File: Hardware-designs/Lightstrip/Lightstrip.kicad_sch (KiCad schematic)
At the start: 22 parts, among them J1 In 24V, J2 lamps, J3 UART, Q1 AO3400A, SW1 PTS526 SM15 SMTR2 LFS, SW2 PTS526 SM15 SMTR2 LFS, U1 TPS560430X3FDBVT, U2 ESP32-WROOM-32E

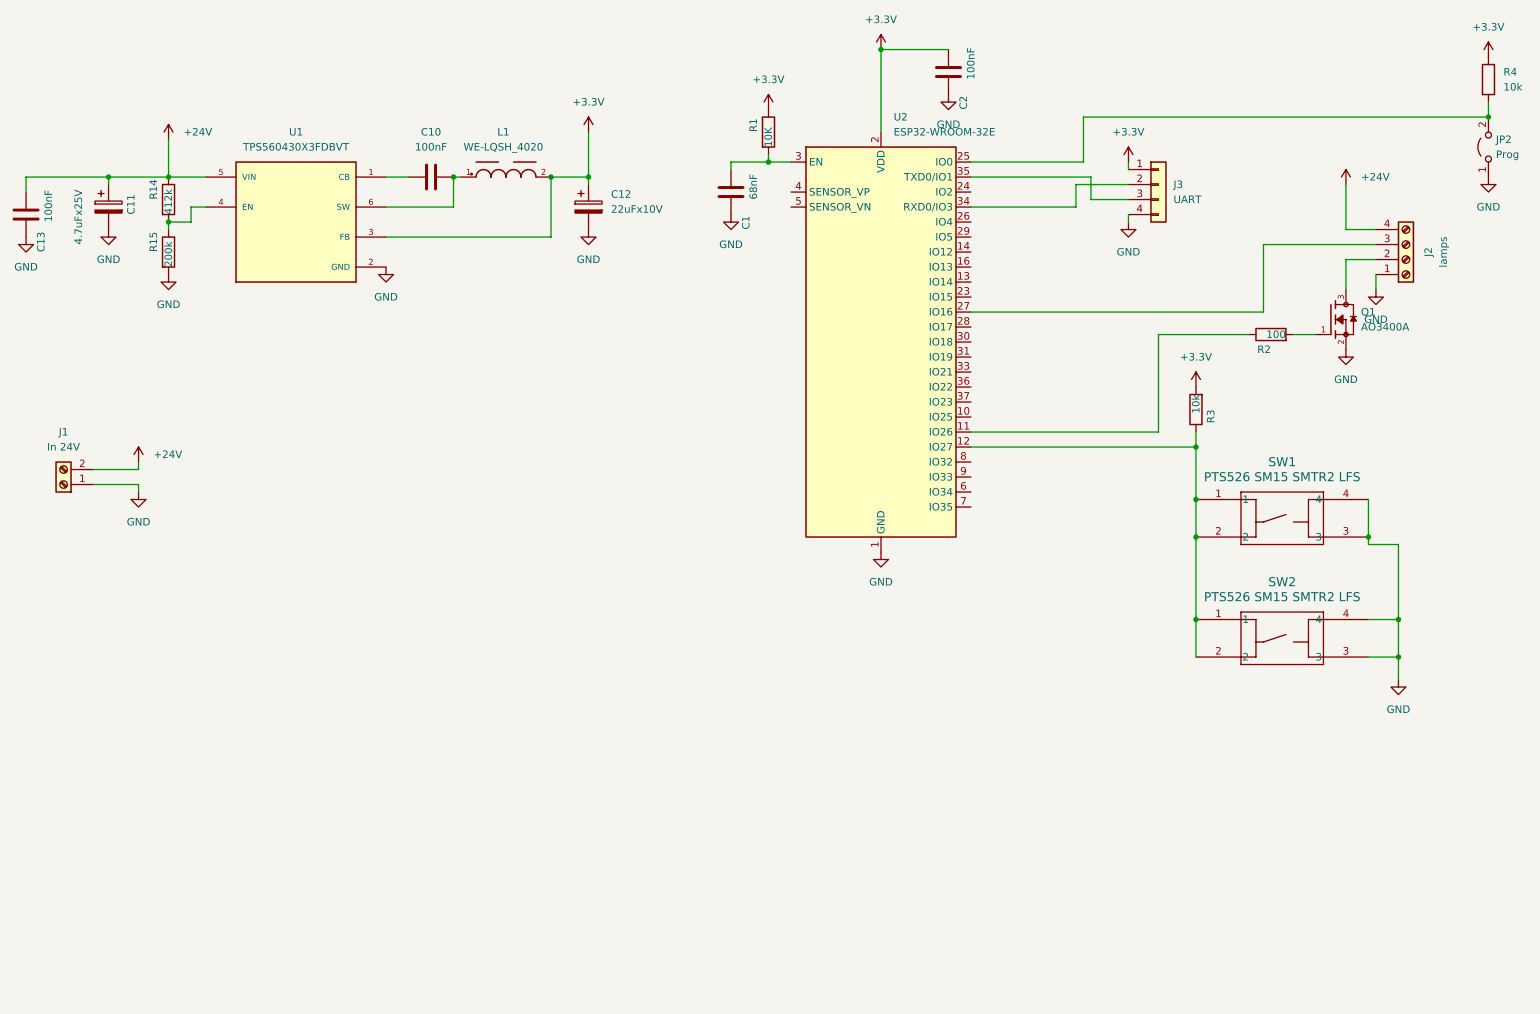
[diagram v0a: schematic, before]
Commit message: Lightstrip version 2
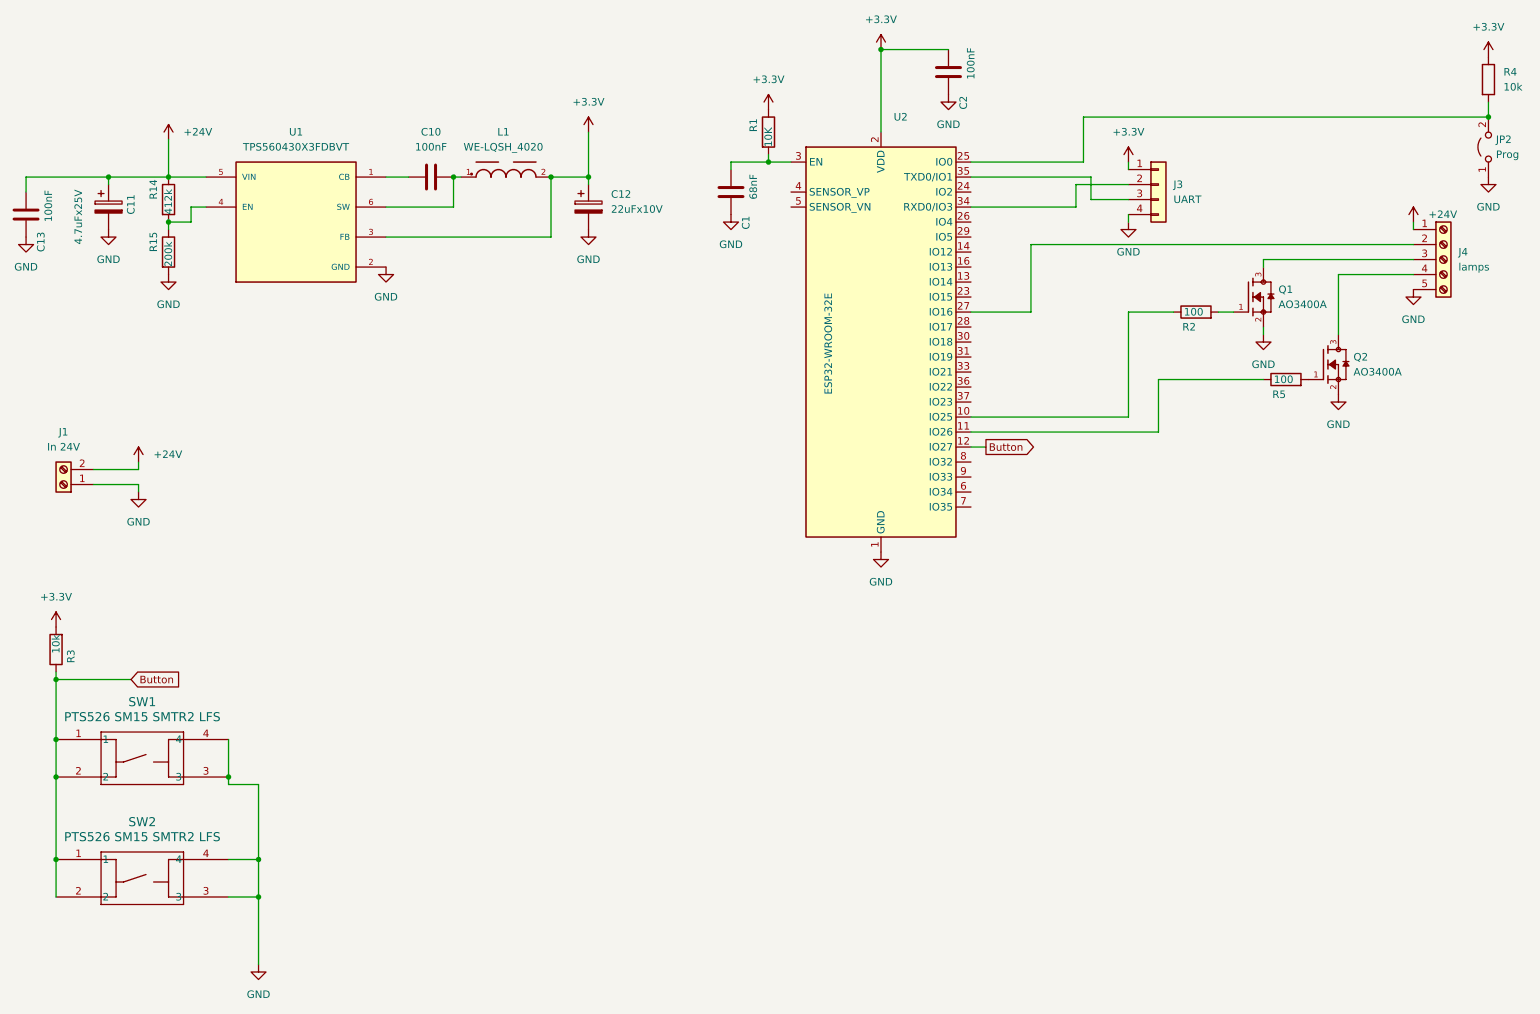
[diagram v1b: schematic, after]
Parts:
- removed J2: lamps, TerminalBlock:TerminalBlock_MaiXu_MX126-5.0-04P_1x04_P5.00mm, symbol Connector:Screw_Terminal_01x04
- added J4: lamps, TerminalBlock:TerminalBlock_MaiXu_MX126-5.0-05P_1x05_P5.00mm, symbol Connector:Screw_Terminal_01x05
- added Q2: AO3400A, AO3400A:SOT95P280X125-3N, symbol AO3400A:AO3400A
- added R5: 100, Resistor_SMD:R_1206_3216Metric_Pad1.30x1.75mm_HandSolder, symbol Device:R
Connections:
- net +24V: now also J4.1 (Pin_1)
- net GND: now also J4.5 (Pin_5), Q2.2
- net Button: now reaches R3.1, SW1.1, SW1.2, SW2.1, SW2.2, U2.12 (IO27)
- net at Q1.3: now also J4.3 (Pin_3)
- net at U2.10 (IO25): now also R2.1
- net at U2.11 (IO26): now also R5.1; no longer R2.1
- net at U2.27 (IO16): now also J4.2 (Pin_2)
- new net: Q2.1, R5.2
- new net: J4.4 (Pin_4), Q2.3
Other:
- title: HueMix-Link Lightstrip Model 5 -> HueMix-Link Lightstrip
- moved on the sheet: Q1, R2, R3, SW1, SW2
